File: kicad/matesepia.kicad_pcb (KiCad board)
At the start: 2 copper layers, 225.3 x 129.3 mm, 63 parts

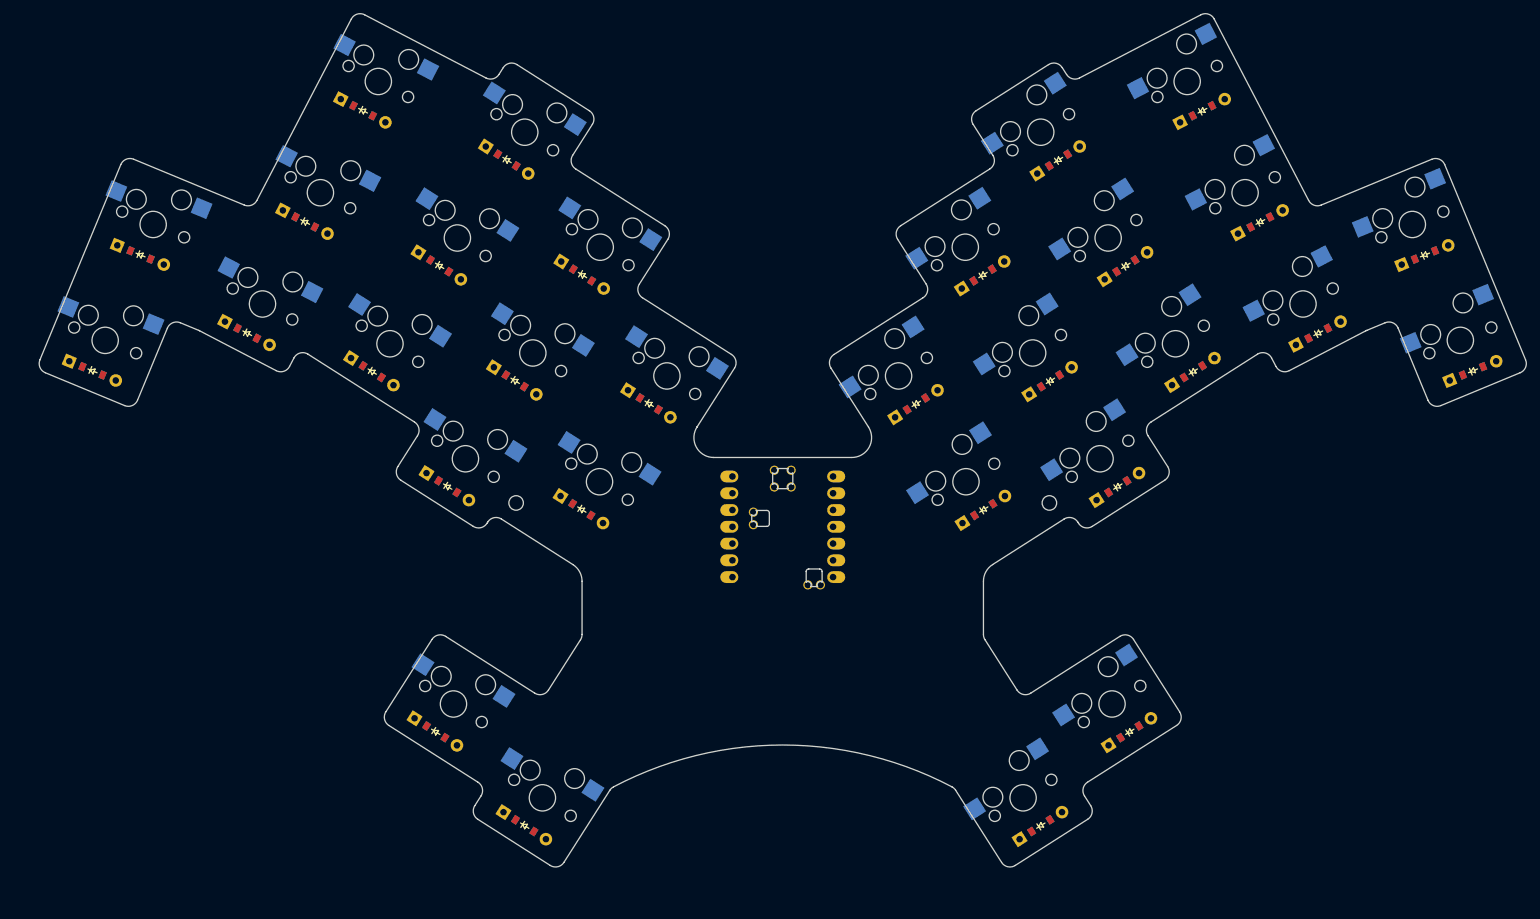
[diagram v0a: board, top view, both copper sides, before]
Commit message: syncing to desktop app
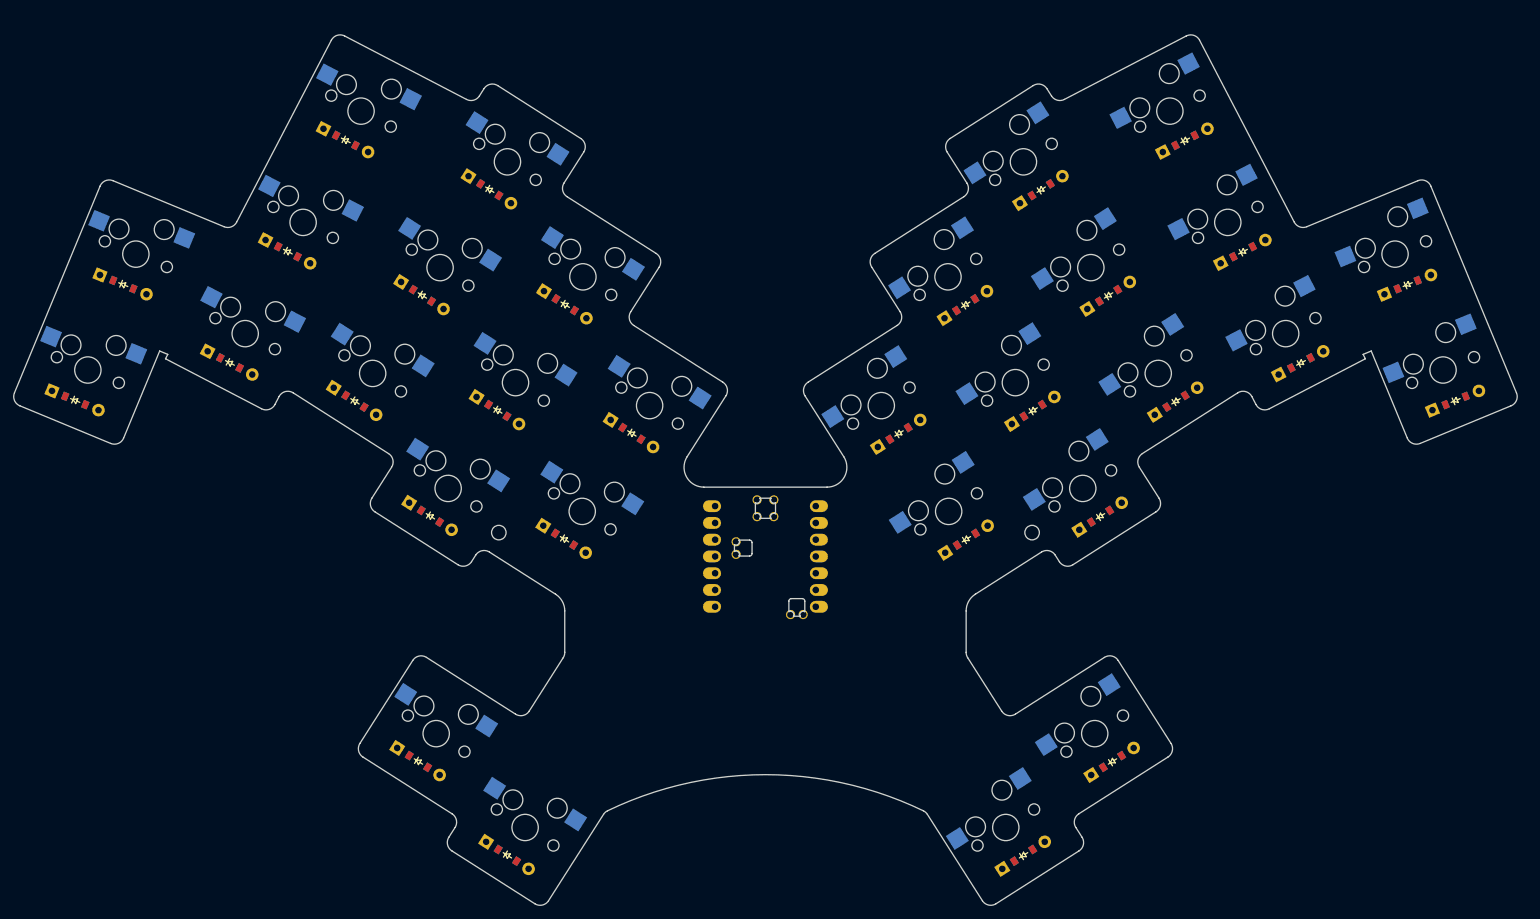
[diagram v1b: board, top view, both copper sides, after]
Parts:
- moved D22 5.20 mm to (197.5, 107.0)
- moved S22 5.20 mm to (194.8, 102.8)
- moved S28 5.20 mm to (110.4, 154.1)
- moved S30 5.20 mm to (183.2, 154.1)
- moved S1 5.20 mm to (44.1, 84.8)
- moved S26 5.20 mm to (164.3, 90.2)
- moved D11 5.20 mm to (116.4, 74.9)
- moved D12 5.20 mm to (116.3, 110.5)
- moved D13 5.20 mm to (126.5, 94.4)
- moved D15 5.20 mm to (244.0, 71.9)
- moved D2 5.20 mm to (49.5, 71.9)
- moved D20 5.20 mm to (198.7, 73.5)
- moved D24 5.20 mm to (177.1, 74.9)
- moved D25 5.20 mm to (177.2, 110.5)
- moved D26 5.20 mm to (167.0, 94.4)
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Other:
- board size 225.3 x 129.3 mm -> 227.7 x 131.8 mm
